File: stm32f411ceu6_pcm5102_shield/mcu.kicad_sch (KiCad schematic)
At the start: 25 parts, among them J100 Conn_01x04_Pin, J101 Conn_01x04_Pin, SW100 RotaryEncoder_Switch_MP, U100 BlackPill, U101 INMP411

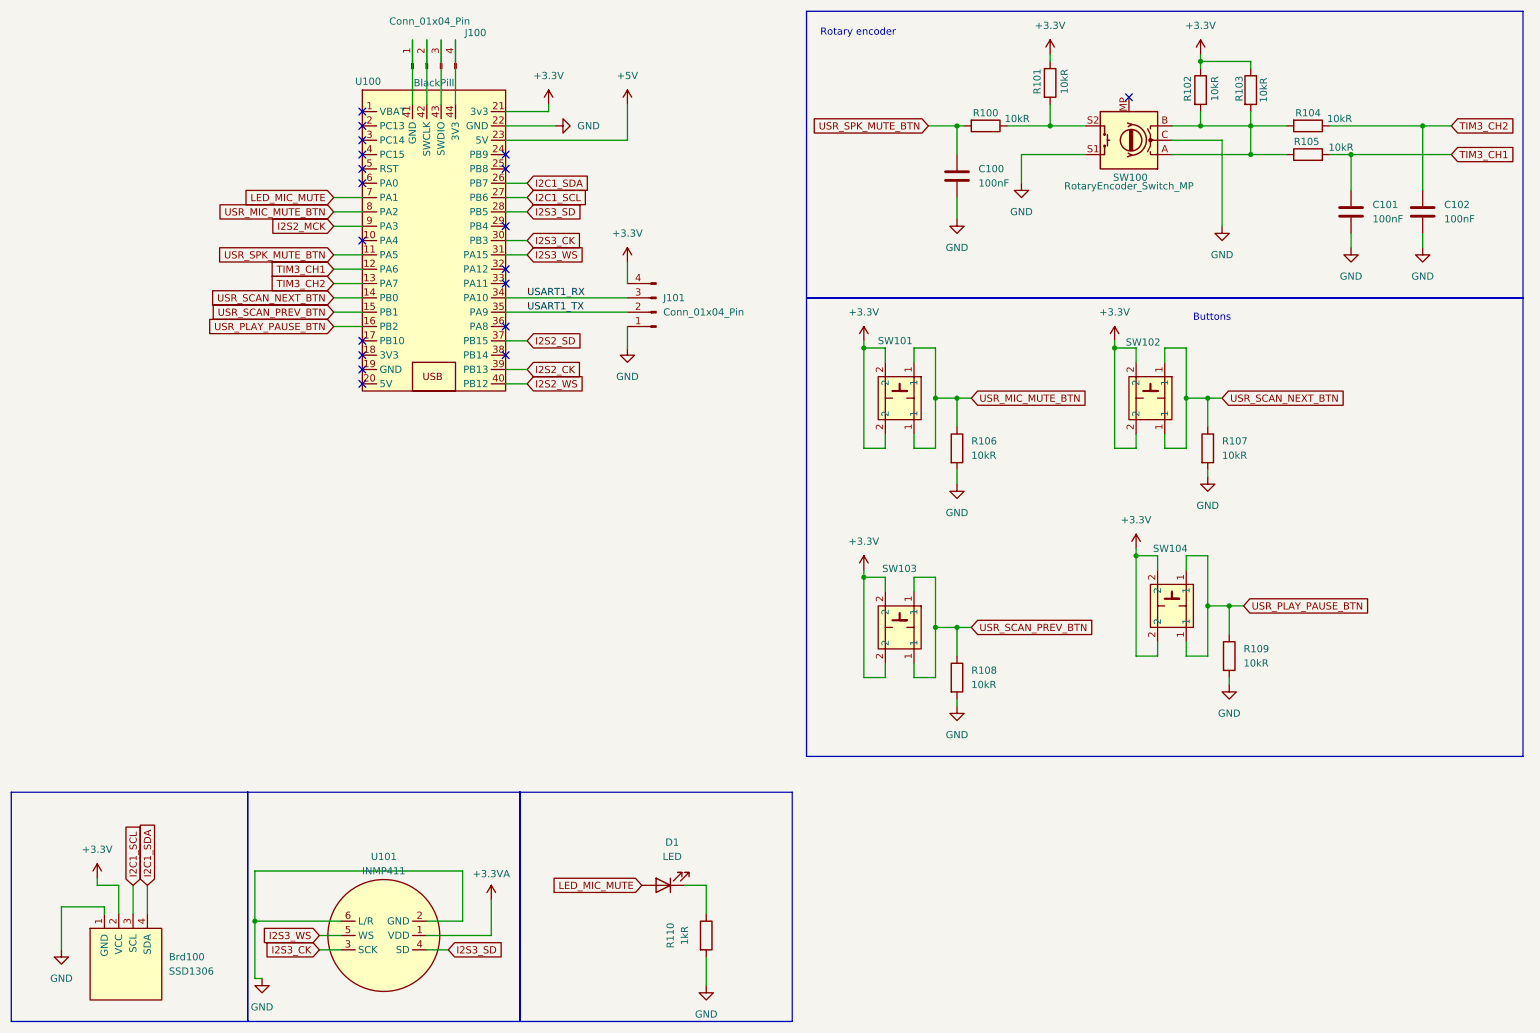
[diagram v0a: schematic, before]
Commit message: Initial layout
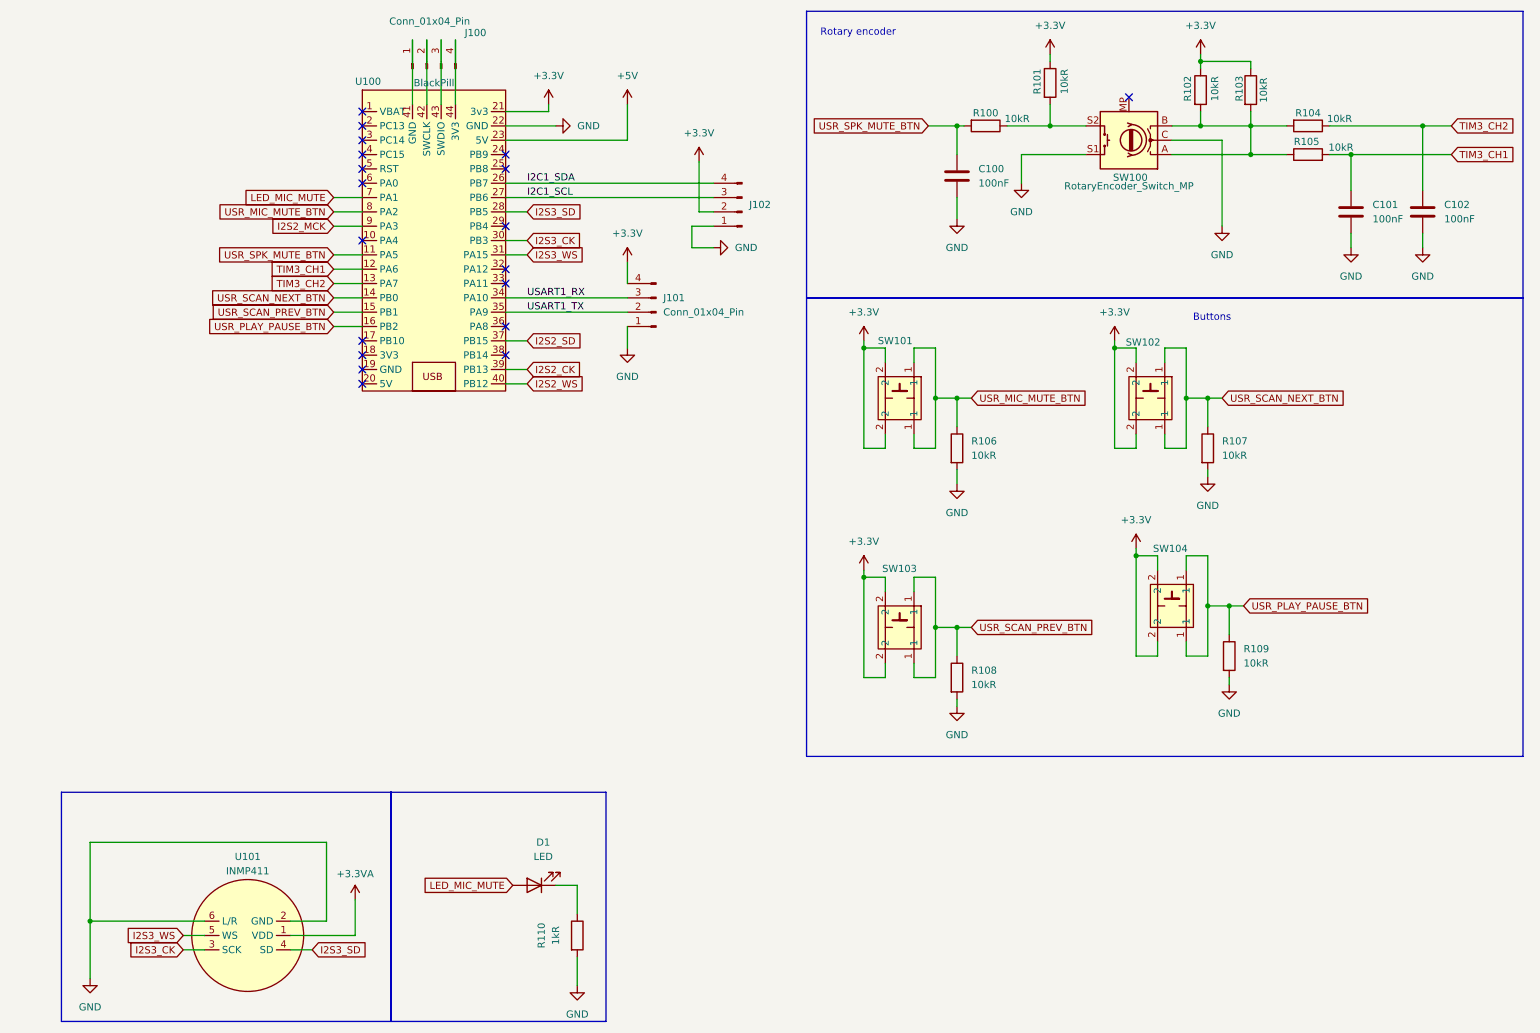
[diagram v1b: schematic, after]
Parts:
- removed Brd100: SSD1306, stm32f401_pcm5102_shiled_lib:128x64OLED, symbol stm32f401_pcm5102_shiled_lib:SSD1306
- added J102: Conn_01x04_Pin, Connector_PinHeader_2.54mm:PinHeader_1x04_P2.54mm_Vertical, symbol Connector:Conn_01x04_Pin
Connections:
- net +3.3V: now also J102.2 (Pin_2)
- net GND: now also J102.1 (Pin_1)
- net I2C1_SCL: now also J102.3 (Pin_3)
- net I2C1_SDA: now also J102.4 (Pin_4)
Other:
- moved on the sheet: D1, R110, U101
